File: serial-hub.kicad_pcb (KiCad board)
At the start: 2 copper layers, 129.5 x 121.9 mm, 43 parts, among them J1 USB_C_Receptacle_USB2.0, J2 RJ45, J3 RJ45, J4 RJ45, J5 RJ45, U1 CH344, U2 AMS1117-3.3, U3 MAX232, U4 MAX232, U5 MAX232, U6 MAX232, Y1 8MHz

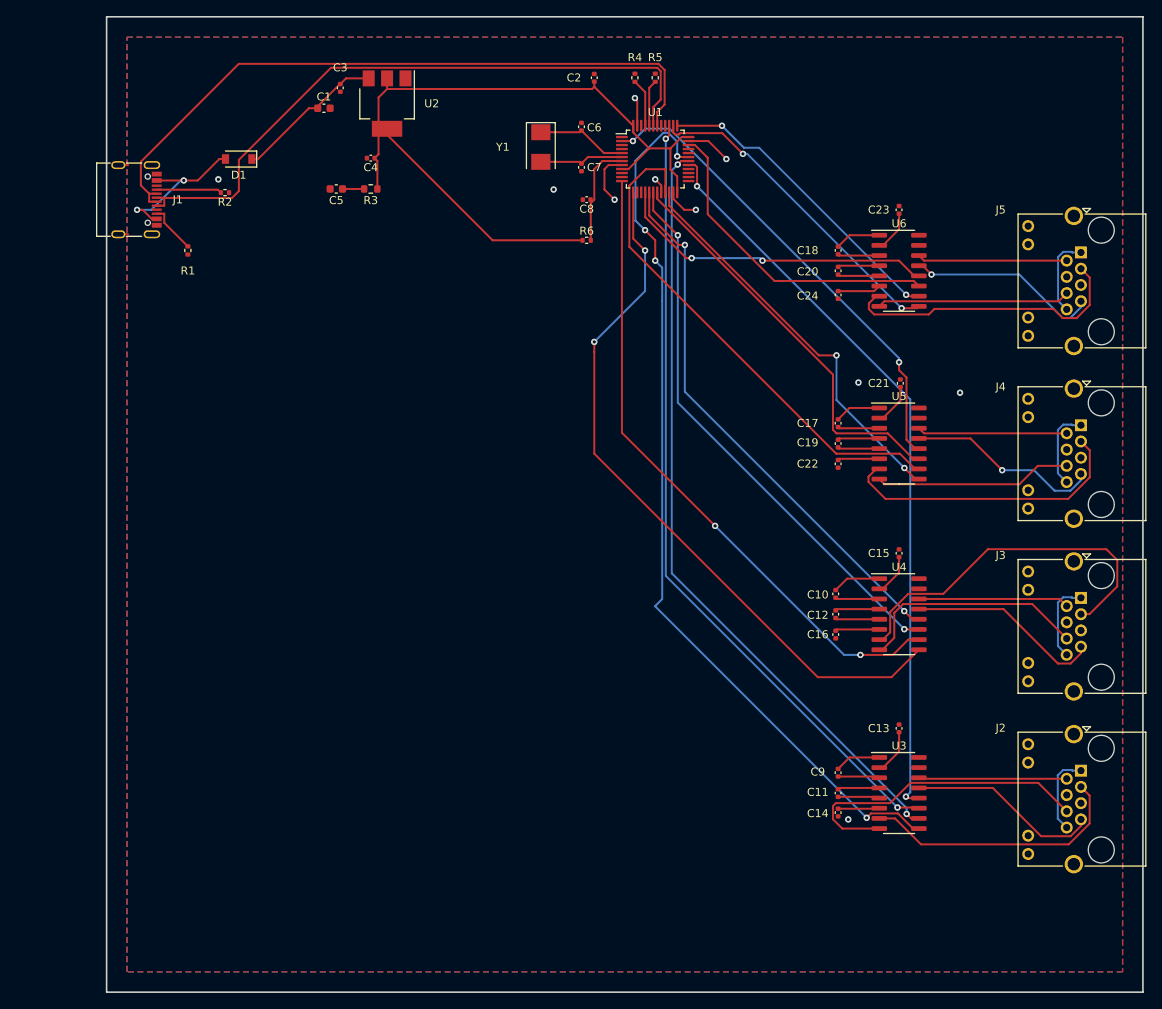
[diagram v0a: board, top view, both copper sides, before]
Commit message: update PCB
Signed-off-by: David Bauer <mail@david-bauer.net>
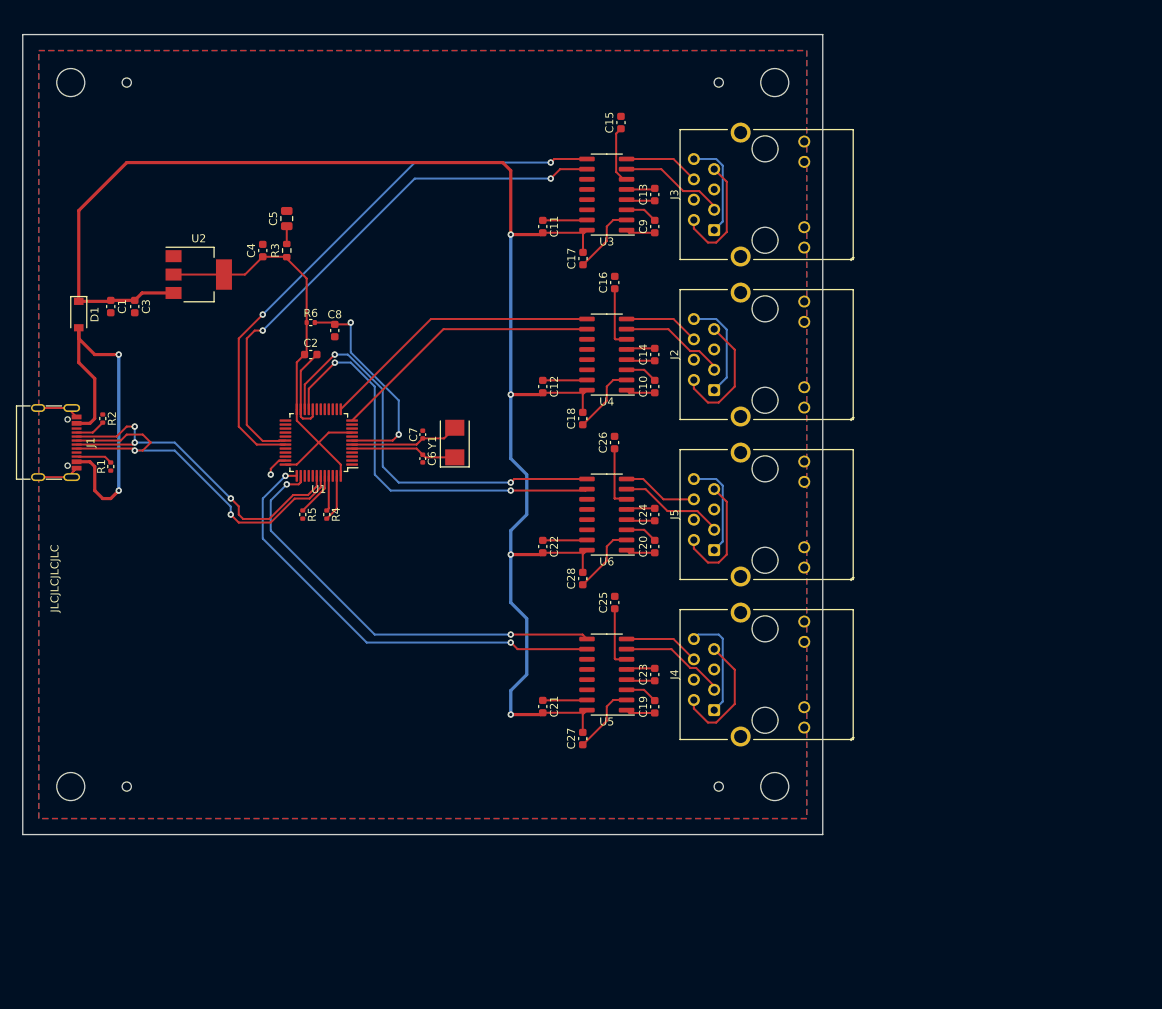
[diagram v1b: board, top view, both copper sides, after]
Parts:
- added C25: 1uF, Capacitor_SMD:C_0603_1608Metric, F.Cu at (94.0, 91.0)
- added C26: 1uF, Capacitor_SMD:C_0603_1608Metric, F.Cu at (94.0, 71.0)
- added C27: 1uF, Capacitor_SMD:C_0603_1608Metric, F.Cu at (90.0, 108.0)
- added C28: 1uF, Capacitor_SMD:C_0603_1608Metric, F.Cu at (90.0, 88.0)
- added REF**: MountingHole_2.1mm, MountingHole:MountingHole_2.1mm, F.Cu at (33.0, 26.0)
- added REF**: MountingHole_2.1mm, MountingHole:MountingHole_2.1mm, F.Cu at (33.0, 114.0)
- added REF**: MountingHole_2.1mm, MountingHole:MountingHole_2.1mm, F.Cu at (107.0, 26.0)
- added REF**: MountingHole_3.5mm, MountingHole:MountingHole_3.5mm, F.Cu at (26.0, 26.0)
- added REF**: MountingHole_2.1mm, MountingHole:MountingHole_2.1mm, F.Cu at (107.0, 114.0)
- added REF**: MountingHole_3.5mm, MountingHole:MountingHole_3.5mm, F.Cu at (114.0, 26.0)
- added REF**: MountingHole_3.5mm, MountingHole:MountingHole_3.5mm, F.Cu at (114.0, 114.0)
- added REF**: MountingHole_3.5mm, MountingHole:MountingHole_3.5mm, F.Cu at (26.0, 114.0)
- C10, C11, C12, C13, C14, C15, C16, C17, C18, C19, C2, C20, C21, C22, C23, C24, C3, C4, C8, C9: footprint Capacitor_SMD:C_0402_1005Metric -> Capacitor_SMD:C_0603_1608Metric
- C5: footprint Capacitor_SMD:C_0603_1608Metric -> Capacitor_SMD:C_0805_2012Metric
- J2, J3, J4, J5: value RJ45 -> RJ45_LED_Shielded; footprint Connector_RJ:RJ45_Amphenol_RJHSE538X -> Connector_RJ:RJ45_Hanrun_HR911105A
- moved U3 83.3 mm to (93.0, 40.0), turned to 180 degrees
- moved C11 79.9 mm to (85.0, 44.0)
- moved C13 73.4 mm to (99.0, 40.0)
- moved C9 72.0 mm to (99.0, 44.0), turned to 90 degrees
- moved R5 70.2 mm to (55.0, 80.0), turned to -90 degrees
- moved R4 66.8 mm to (58.0, 80.0), turned to -90 degrees
- moved J2 66.1 mm to (106.4, 64.4), turned to 90 degrees
- moved C23 65.6 mm to (99.0, 100.0)
- moved J3 64.9 mm to (106.4, 44.4), turned to 90 degrees
- moved C15 64.1 mm to (94.8, 31.0)
- moved C14 61.7 mm to (99.0, 60.0), turned to 90 degrees
- moved C21 60.3 mm to (85.0, 104.0), turned to -90 degrees
- moved J5 59.0 mm to (106.4, 84.4), turned to 90 degrees
- moved J4 58.1 mm to (106.4, 104.4), turned to 90 degrees
- moved U1 55.0 mm to (57.0, 71.0), turned to 180 degrees
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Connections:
- C11 pad 1: Net-(C11-Pad1) -> GND
- C11 pad 2: Net-(C11-Pad2) -> VBUS
- C12 pad 1: Net-(C12-Pad1) -> GND
- C12 pad 2: Net-(C12-Pad2) -> VBUS
- C13 pad 2: GND -> Net-(C13-Pad2)
- C14 pad 2: GND -> Net-(C14-Pad2)
- C17 pad 2: Net-(C17-Pad2) -> VBUS
- C18 pad 2: Net-(C18-Pad2) -> VBUS
- C21 pad 1: Net-(C21-Pad1) -> GND
- C21 pad 2: GND -> VBUS
- C22 pad 1: Net-(C22-Pad1) -> GND
- C22 pad 2: GND -> VBUS
- C23 pad 2: GND -> Net-(C23-Pad2)
- C24 pad 2: GND -> Net-(C24-Pad2)
- J2 pad 10: (no net) -> unconnected-(J2-Pad10)
- J2 pad 11: (no net) -> unconnected-(J2-Pad11)
- J2 pad 12: (no net) -> unconnected-(J2-Pad12)
- J2 pad 2: /P0_DTR -> Net-(J2-Pad2)
- J2 pad 3: /P0_TX -> /P1_TX
- J2 pad 6: /P0_RX -> /P1_RX
- J2 pad 7: /P0_DSR -> Net-(J2-Pad2)
- J2 pad 9: (no net) -> unconnected-(J2-Pad9)
- J2 pad SH: (no net) -> GND
- J3 pad 10: (no net) -> unconnected-(J3-Pad10)
- J3 pad 11: (no net) -> unconnected-(J3-Pad11)
- J3 pad 12: (no net) -> unconnected-(J3-Pad12)
- J3 pad 2: /P1_DTR -> Net-(J3-Pad2)
- J3 pad 3: /P1_TX -> /P0_TX
- J3 pad 6: /P1_RX -> /P0_RX
- J3 pad 7: /P1_DSR -> Net-(J3-Pad2)
- J3 pad 9: (no net) -> unconnected-(J3-Pad9)
- J3 pad SH: (no net) -> GND
- J4 pad 10: (no net) -> unconnected-(J4-Pad10)
- J4 pad 11: (no net) -> unconnected-(J4-Pad11)
- J4 pad 12: (no net) -> unconnected-(J4-Pad12)
- J4 pad 2: /P2_DTR -> Net-(J4-Pad2)
- J4 pad 3: /P2_TX -> /P3_TX
- J4 pad 6: /P2_RX -> /P3_RX
- J4 pad 7: /P2_DSR -> Net-(J4-Pad2)
- J4 pad 9: (no net) -> unconnected-(J4-Pad9)
- J4 pad SH: (no net) -> GND
- J5 pad 10: (no net) -> unconnected-(J5-Pad10)
- J5 pad 11: (no net) -> unconnected-(J5-Pad11)
- J5 pad 12: (no net) -> unconnected-(J5-Pad12)
- J5 pad 2: /P3_DTR -> Net-(J5-Pad2)
- J5 pad 3: /P3_TX -> /P2_TX
- J5 pad 6: /P3_RX -> /P2_RX
- J5 pad 7: /P3_DSR -> Net-(J5-Pad2)
- J5 pad 9: (no net) -> unconnected-(J5-Pad9)
- J5 pad SH: (no net) -> GND
- U1 pad 16: /C3_DSR -> unconnected-(U1-Pad16)
- U1 pad 17: /C1_DSR -> unconnected-(U1-Pad17)
- U1 pad 18: /C1_DTR -> unconnected-(U1-Pad18)
- U1 pad 19: /C2_DTR -> unconnected-(U1-Pad19)
- U1 pad 2: /C2_DSR -> unconnected-(U1-Pad2)
- U1 pad 29: /C0_DSR -> unconnected-(U1-Pad29)
- U1 pad 34: /C3_DTR -> unconnected-(U1-Pad34)
- U1 pad 39: /C0_DTR -> unconnected-(U1-Pad39)
- U3 pad 11: /C0_DTR -> unconnected-(U3-Pad11)
- U3 pad 12: /C0_DSR -> unconnected-(U3-Pad12)
- U3 pad 13: /P0_DSR -> unconnected-(U3-Pad13)
- U3 pad 14: /P0_DTR -> unconnected-(U3-Pad14)
- U3 pad 16: unconnected-(U3-Pad16) -> VBUS
- U3 pad 2: Net-(C13-Pad1) -> Net-(C17-Pad1)
- U3 pad 4: Net-(C11-Pad1) -> Net-(C13-Pad1)
- U3 pad 5: Net-(C11-Pad2) -> Net-(C13-Pad2)
- U3 pad 6: Net-(C14-Pad1) -> Net-(C15-Pad1)
- U4 pad 11: /C1_DTR -> unconnected-(U4-Pad11)
- U4 pad 12: /C1_DSR -> unconnected-(U4-Pad12)
- U4 pad 13: /P1_DSR -> unconnected-(U4-Pad13)
- U4 pad 14: /P1_DTR -> unconnected-(U4-Pad14)
- U4 pad 16: unconnected-(U4-Pad16) -> VBUS
- U4 pad 2: Net-(C15-Pad1) -> Net-(C18-Pad1)
- U4 pad 4: Net-(C12-Pad1) -> Net-(C14-Pad1)
- U4 pad 5: Net-(C12-Pad2) -> Net-(C14-Pad2)
- U5 pad 1: Net-(C17-Pad1) -> Net-(C19-Pad1)
- U5 pad 10: /C2_TX -> /C3_TX
- U5 pad 11: /C2_DTR -> unconnected-(U5-Pad11)
- U5 pad 12: /C2_DSR -> unconnected-(U5-Pad12)
- U5 pad 13: /P2_DSR -> unconnected-(U5-Pad13)
- U5 pad 14: /P2_DTR -> unconnected-(U5-Pad14)
- U5 pad 16: unconnected-(U5-Pad16) -> VBUS
- U5 pad 2: Net-(C21-Pad1) -> Net-(C27-Pad1)
- U5 pad 3: Net-(C17-Pad2) -> Net-(C19-Pad2)
- U5 pad 4: Net-(C19-Pad1) -> Net-(C23-Pad1)
- U5 pad 5: Net-(C19-Pad2) -> Net-(C23-Pad2)
- U5 pad 6: Net-(C22-Pad1) -> Net-(C25-Pad1)
- U5 pad 7: /P2_TX -> /P3_TX
- U5 pad 8: /P2_RX -> /P3_RX
- U5 pad 9: /C2_RX -> /C3_RX
- U6 pad 1: Net-(C18-Pad1) -> Net-(C20-Pad1)
- U6 pad 10: /C3_TX -> /C2_TX
- U6 pad 11: /C3_DTR -> unconnected-(U6-Pad11)
- U6 pad 12: /C3_DSR -> unconnected-(U6-Pad12)
- U6 pad 13: /P3_DSR -> unconnected-(U6-Pad13)
- U6 pad 14: /P3_DTR -> unconnected-(U6-Pad14)
- U6 pad 16: unconnected-(U6-Pad16) -> VBUS
- U6 pad 2: Net-(C23-Pad1) -> Net-(C28-Pad1)
- U6 pad 3: Net-(C18-Pad2) -> Net-(C20-Pad2)
- U6 pad 4: Net-(C20-Pad1) -> Net-(C24-Pad1)
- U6 pad 5: Net-(C20-Pad2) -> Net-(C24-Pad2)
- U6 pad 6: Net-(C24-Pad1) -> Net-(C26-Pad1)
- U6 pad 7: /P3_TX -> /P2_TX
- U6 pad 8: /P3_RX -> /P2_RX
- U6 pad 9: /C3_RX -> /C2_RX
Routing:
- net VBUS: track 18.9 -> 202.8 mm, vias 0 -> 4
- net /C0_DTR: track 100.1 -> 0.00 mm, vias 2 -> 0
- net /C0_DSR: track 92.5 -> 0.00 mm, vias 2 -> 0
- net /C1_DTR: track 69.4 -> 0.00 mm, vias 2 -> 0
- net /C1_DSR: track 68.3 -> 0.00 mm, vias 2 -> 0
- net /C2_DSR: track 59.7 -> 0.00 mm, vias 2 -> 0
- net /C1_RX: track 89.5 -> 35.4 mm, vias 2 -> 0
- net /C2_DTR: track 51.0 -> 0.00 mm
- net /C1_TX: track 80.9 -> 34.1 mm, vias 2 -> 0
- net +3.3V: track 99.4 -> 56.2 mm
- net /C0_RX: track 112.8 -> 70.6 mm, vias 4 -> 2
- net /C3_DSR: track 40.3 -> 0.00 mm, vias 2 -> 0
- net /C3_DTR: track 40.2 -> 0.00 mm
- net /HOST_DM: track 85.5 -> 47.5 mm, vias 0 -> 3
- net /P1_TX: track 45.7 -> 13.3 mm
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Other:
- board size 129.5 x 121.9 mm -> 100 x 100 mm
- board text added: "JLCJLCJLCJLC"
